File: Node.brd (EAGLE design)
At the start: 38.1 x 38.1 mm, 65 parts, among them J1 DF12A3.0-14DS, Q1 16MHz, U1 ATMEGA32U4QFN, U2 NRF24L01NOPAD, U3 LTC3553, U4 L3GD20, U6 LSM303DLHC, U7 BD2425NNRF0404, U9 RCLAMP0502A, X1 USBSMD

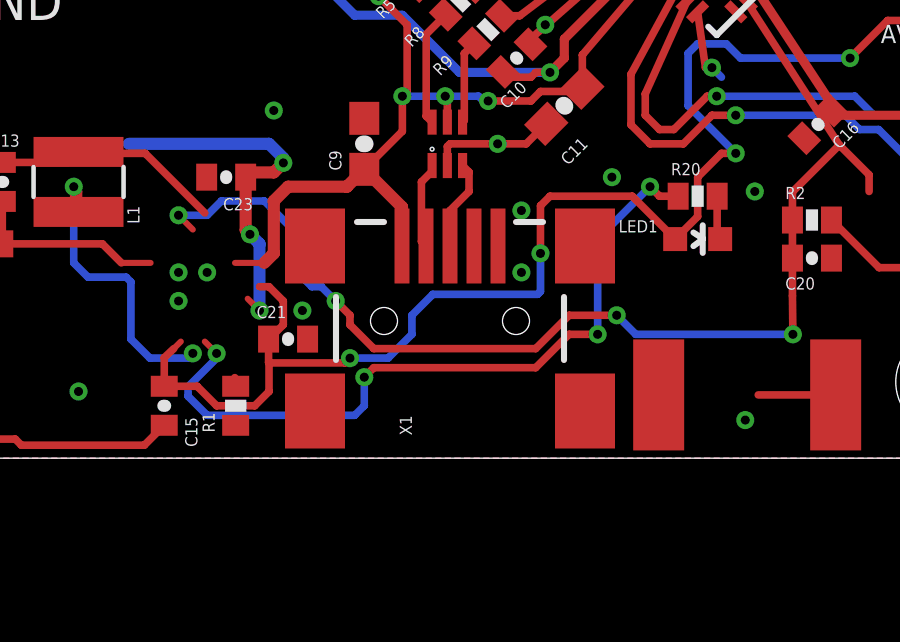
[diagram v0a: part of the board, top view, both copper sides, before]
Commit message: usb port parts
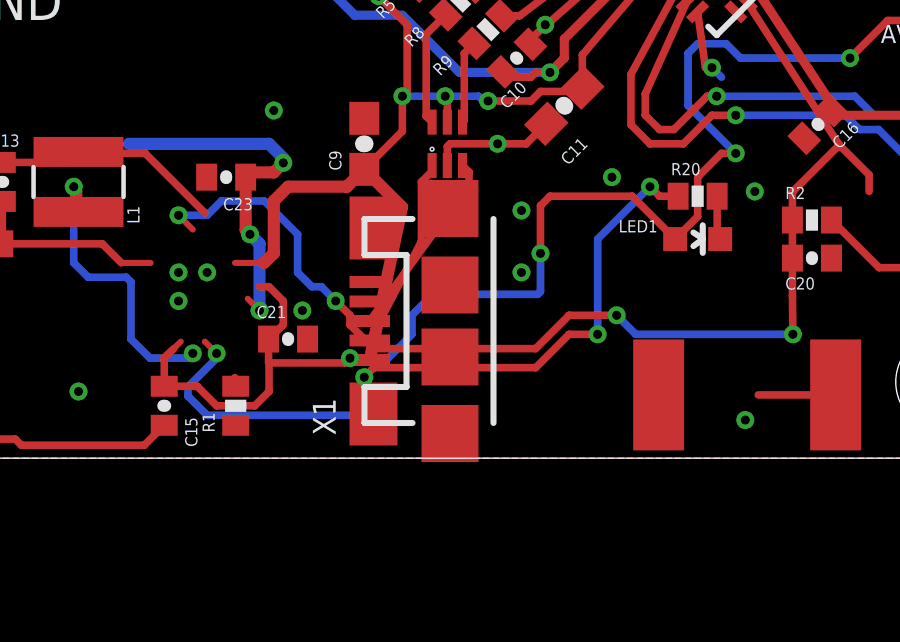
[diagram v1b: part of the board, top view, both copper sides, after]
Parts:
- X1: value USBSMD -> USB-FCI; device SparkFun:USB-MINIB -> adjacent-reality:USB-MICROB-FCI
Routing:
- net VBUS: track 43.9 -> 47.8 mm
- net D-: track 2.89 -> 6.40 mm
- net D+: track 3.03 -> 6.40 mm
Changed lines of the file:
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@@
 <attribute name="VALUE" x="18.4785" y="32.258" size="0.4064" layer="27" font="vector" rot="R180"/>
 </element>
-<element name="X1" library="SparkFun" package="USB-MINIB" value="USBSMD" x="19.05" y="4.572" rot="R90"/>
+<element name="X1" library="adjacent-reality" package="USB-MICROB-FCI" value="USB-FCI" x="19.05" y="4.572" rot="R90"/>
 <element name="C9" library="SparkFun" package="0603-CAP" value="10uF" x="16.1925" y="10.4775" rot="R90"/>
 <element name="C10" library="SparkFun" package="0402-CAP" value="1uF" x="21.2725" y="13.335" smashed="yes" rot="R45">
@@
 <wire x1="18.9611" y1="10.3886" x2="16.1925" y2="11.3275" width="0" layer="19" extent="1-1"/>
 <wire x1="21.43125" y1="8.255" x2="21.59" y2="10.4775" width="0" layer="19" extent="1-1"/>
-<wire x1="20.65" y1="7.072" x2="21.43125" y2="8.255" width="0" layer="19" extent="1-1"/>
-<wire x1="21.43125" y1="6.19125" x2="20.65" y2="7.072" width="0" layer="19" extent="1-1"/>
+<wire x1="16.375" y1="5.872" x2="21.43125" y2="8.255" width="0" layer="19" extent="1-1"/>
+<wire x1="21.43125" y1="6.19125" x2="16.375" y2="5.872" width="0" layer="19" extent="1-1"/>
 <wire x1="21.73211875" y1="13.79461875" x2="22.25895625" y2="11.14645625" width="0" layer="19" extent="1-1"/>
 <wire x1="22.225" y1="14.44625" x2="21.73211875" y2="13.973490625" width="0" layer="19" extent="1-1"/>
@@
 <wire x1="25.8893875" y1="16.29228125" x2="23.461040625" y2="13.43966875" width="0.254" layer="1"/>
 <wire x1="23.461040625" y1="13.43966875" x2="23.461040625" y2="12.348540625" width="0.254" layer="1"/>
-<wire x1="17.45" y1="7.072" x2="17.45" y2="8.37" width="0.4064" layer="1"/>
+<wire x1="16.375" y1="3.272" x2="17.45" y2="8.37" width="0.4064" layer="1"/>
 <wire x1="17.45" y1="8.37" x2="16.1925" y2="9.6275" width="0.4064" layer="1"/>
 <wire x1="13.6525" y1="9.04875" x2="15.61375" y2="9.04875" width="0.4064" layer="1"/>
@@
 <contactref element="X1" pad="D-"/>
 <contactref element="U9" pad="1"/>
-<wire x1="18.25" y1="7.072" x2="18.0975" y2="7.2245" width="0.254" layer="1"/>
+<wire x1="16.375" y1="3.922" x2="18.0975" y2="7.2245" width="0.254" layer="1"/>
 <wire x1="18.0975" y1="7.2245" x2="18.0975" y2="9.2075" width="0.254" layer="1"/>
 <wire x1="18.0975" y1="9.2075" x2="18.4531" y2="9.5631" width="0.254" layer="1"/>
@@
 <contactref element="X1" pad="D+"/>
 <contactref element="U9" pad="3"/>
-<wire x1="19.05" y1="7.072" x2="19.05" y2="8.255" width="0.254" layer="1"/>
+<wire x1="16.375" y1="4.572" x2="19.05" y2="8.255" width="0.254" layer="1"/>
 <wire x1="19.05" y1="8.255" x2="19.685" y2="8.89" width="0.254" layer="1"/>
 <wire x1="19.685" y1="8.89" x2="19.685" y2="9.5377" width="0.254" layer="1"/>
